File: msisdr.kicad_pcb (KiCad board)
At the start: 2 copper layers, 46.3 x 90.7 mm, 82 parts, among them J1 VCC_GPIO, J10 SMA_VHF1, J11 USB_OTG, J2 GPIO0, J3 GPIO1, J4 GPIO2, J5 GPIO3, J6 SMA_0_30MHZ, J7 SMA_30_60MHZ, J8 SMA_VHF2, J9 SMA_UHF, U1 msi2500, U2 msi001, U3 RT9193-28, U4 AP7313-30SAG, Y1 24MHz, Y2 24MHZ

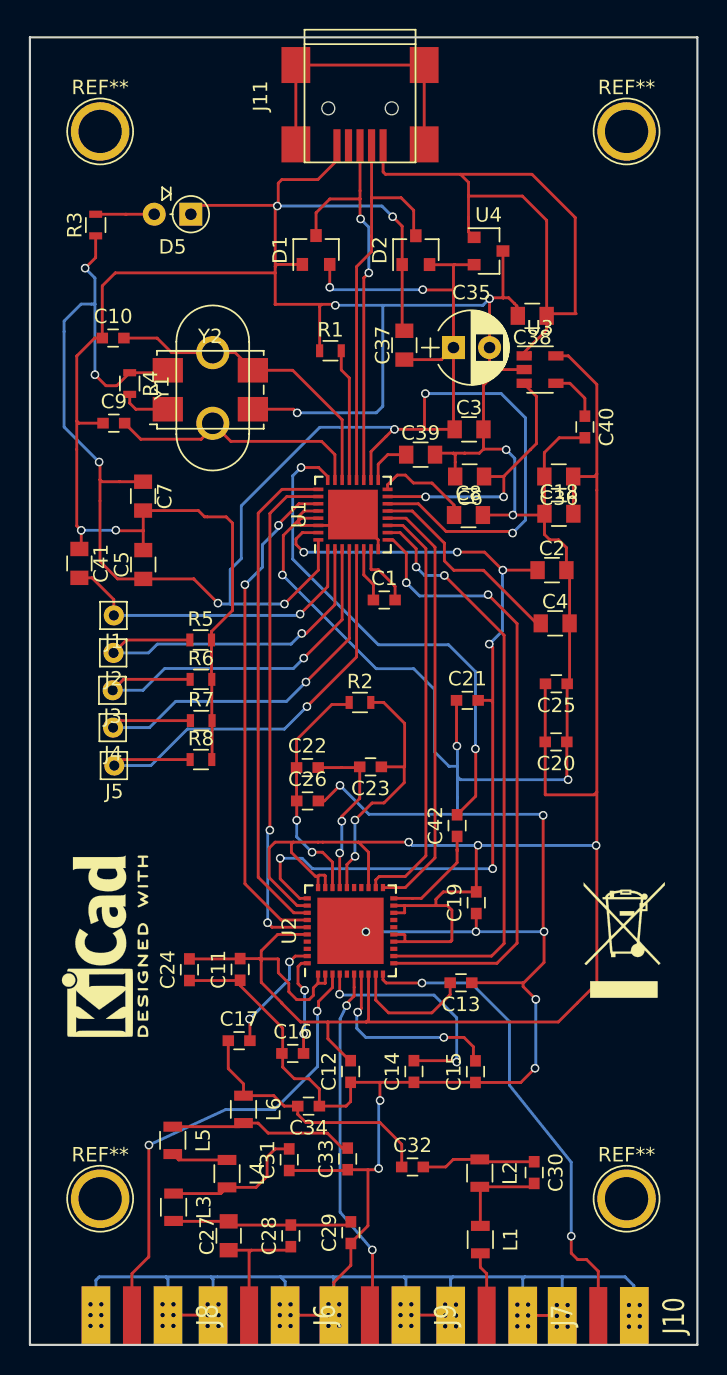
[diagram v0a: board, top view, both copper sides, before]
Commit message: finish route and output gerber file
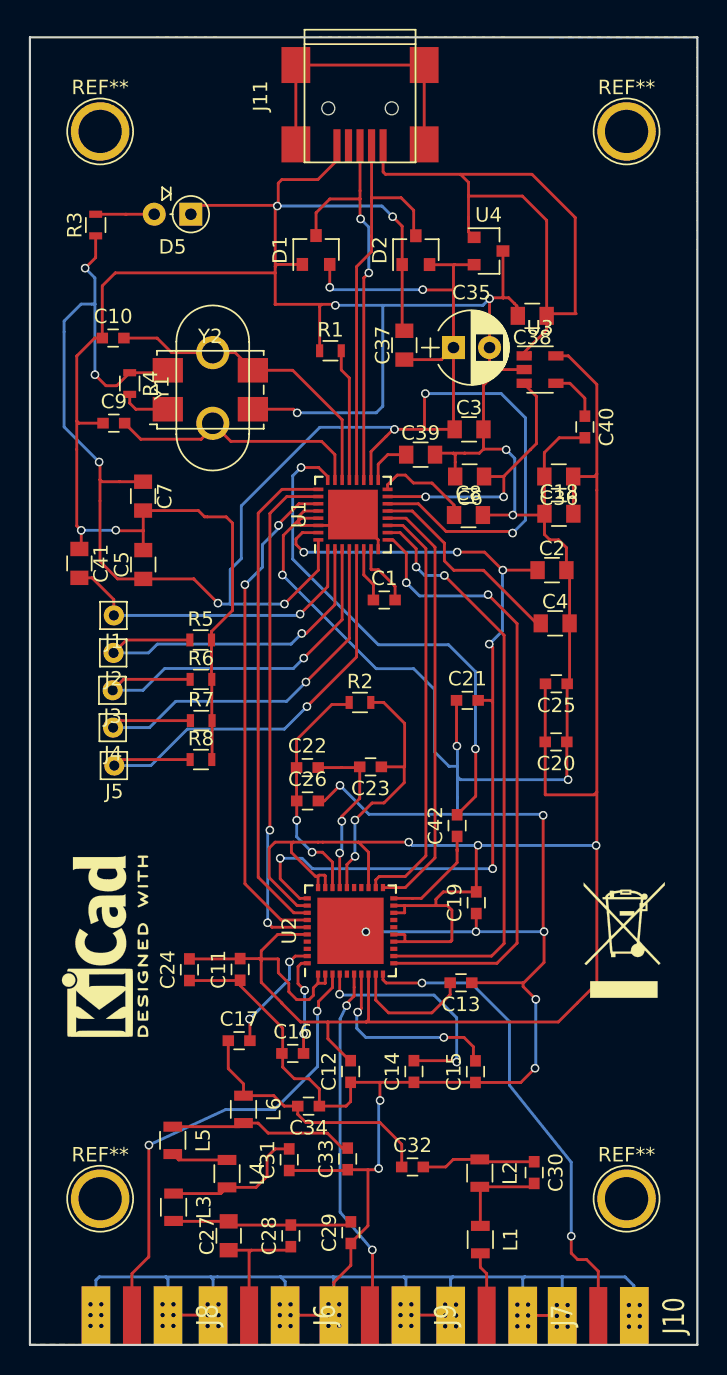
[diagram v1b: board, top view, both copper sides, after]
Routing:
- added copper zone on B.Cu, net GND
- added copper zone on F.Cu, net GND
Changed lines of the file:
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@@
     (visible_elements 7FFEFFFF)
     (pcbplotparams
-      (layerselection 0x00030_80000001)
+      (layerselection 0x01fff_80000001)
       (usegerberextensions false)
       (excludeedgelayer true)
@@
       (outputformat 1)
       (mirror false)
-      (drillshape 1)
+      (drillshape 0)
       (scaleselection 1)
-      (outputdirectory ""))
+      (outputdirectory gerber/))
   )
   (net 0 "")
@@
   (segment (start 125.01 71.34) (end 120.813 71.34) (width 0.2) (layer F.Cu) (net 7))
   (segment (start 125.799 70.226) (end 125.809 70.236) (width 0.2) (layer F.Cu) (net 7))
-  (segment (start 144.079 102.726) (end 144.079 99.611) (width 0.2) (layer F.Cu) (net 8) (status 400000))
+  (segment (start 144.079 102.726) (end 144.079 99.611) (width 0.2) (layer F.Cu) (net 8))
   (segment (start 144.14 99.43) (end 144.14 99.506) (width 0.2) (layer B.Cu) (net 8))
   (segment (start 144.184 99.474) (end 144.14 99.43) (width 0.2) (layer B.Cu) (net 8))
@@
   (segment (start 142.75 100.7) (end 140.274 103.176) (width 0.2) (layer F.Cu) (net 22))
   (segment (start 142.75 99.9) (end 142.75 99.78) (width 0.2) (layer F.Cu) (net 22))
-  (segment (start 142.75 99.78) (end 142.75 98.88) (width 0.2) (layer F.Cu) (net 22) (status 800000))
+  (segment (start 142.75 99.78) (end 142.75 98.88) (width 0.2) (layer F.Cu) (net 22))
   (segment (start 132.359 104.176) (end 131.429 104.176) (width 0.2) (layer F.Cu) (net 23))
   (segment (start 130.609 74.816) (end 133.129 74.816) (width 0.2) (layer F.Cu) (net 23))
@@
   (segment (start 123.09094 123.64208) (end 126.36762 123.64208) (width 0.2) (layer F.Cu) (net 33))
   (segment (start 126.36762 123.64208) (end 126.7968 123.2129) (width 0.2) (layer F.Cu) (net 33))
-  (segment (start 116.689 77.656) (end 116.689 78.821) (width 0.2) (layer F.Cu) (net 34) (status 800000))
-  (segment (start 116.689 78.821) (end 116.56 78.95) (width 0.2) (layer F.Cu) (net 34) (status C00000))
+  (segment (start 116.689 77.656) (end 116.689 78.821) (width 0.2) (layer F.Cu) (net 34))
+  (segment (start 116.689 78.821) (end 116.56 78.95) (width 0.2) (layer F.Cu) (net 34))
   (segment (start 138.94 59.23) (end 138.94 63.67) (width 0.2) (layer F.Cu) (net 34))
   (segment (start 138.94 63.67) (end 139.09 63.82) (width 0.2) (layer F.Cu) (net 34))
@@
   (segment (start 120.05 68.84) (end 120.05 68.23) (width 0.2) (layer F.Cu) (net 61))
   (segment (start 120.47 69.26) (end 120.05 68.84) (width 0.2) (layer F.Cu) (net 61))
-  (segment (start 116.56 80.95) (end 117.44 80.95) (width 0.2) (layer F.Cu) (net 62) (status 400000))
-  (segment (start 118.949 82.459) (end 118.949 83.556) (width 0.2) (layer F.Cu) (net 62) (status 800000))
+  (segment (start 116.56 80.95) (end 117.44 80.95) (width 0.2) (layer F.Cu) (net 62))
+  (segment (start 118.949 82.459) (end 118.949 83.556) (width 0.2) (layer F.Cu) (net 62))
   (segment (start 117.44 80.95) (end 118.949 82.459) (width 0.2) (layer F.Cu) (net 62))
   (segment (start 118.949 83.556) (end 131.779 83.556) (width 0.2) (layer B.Cu) (net 62))
@@
   (via (at 131.869 83.466) (size 0.6) (drill 0.4) (layers F.Cu B.Cu) (net 62))
   (segment (start 131.779 83.556) (end 131.869 83.466) (width 0.2) (layer B.Cu) (net 62))
-  (segment (start 133.779 74.166) (end 133.779 73.929) (width 0.2) (layer F.Cu) (net 63) (status C00000))
-  (segment (start 133.779 73.929) (end 133.15 73.3) (width 0.2) (layer F.Cu) (net 63) (status 400000))
+  (segment (start 133.779 74.166) (end 133.779 73.929) (width 0.2) (layer F.Cu) (net 63))
+  (segment (start 133.779 73.929) (end 133.15 73.3) (width 0.2) (layer F.Cu) (net 63))
   (segment (start 133.15 73.3) (end 131.93 73.3) (width 0.2) (layer F.Cu) (net 63))
   (via (at 131.93 73.3) (size 0.6) (drill 0.4) (layers F.Cu B.Cu) (net 63))
@@
   (segment (start 144.02 92.81) (end 144.04 92.83) (width 0.2) (layer F.Cu) (net 63))
   (segment (start 144.04 92.83) (end 144.04 96.09) (width 0.2) (layer F.Cu) (net 63))
-  (segment (start 144.04 96.09) (end 142.75 97.38) (width 0.2) (layer F.Cu) (net 63) (status 800000))
+  (segment (start 144.04 96.09) (end 142.75 97.38) (width 0.2) (layer F.Cu) (net 63))
+  (zone (net 34) (net_name GND) (layer F.Cu) (hatch edge 0.508)
+    (connect_pads (clearance 0.508))
+    (min_thickness 0.254)
+    (fill yes (arc_segments 16) (thermal_gap 0.508) (thermal_bridge_width 0.508))
+    (polygon
+      (pts
+        (xy 113.16 43.47) (xy 113.15 134.1) (xy 159.41 134.12) (xy 159.39 43.46) (xy 113.17 43.47)
+      )
+    )
+  )
+  (zone (net 34) (net_name GND) (layer B.Cu) (hatch edge 0.508)
+    (connect_pads (clearance 0.508))
+    (min_thickness 0.254)
+    (fill yes (arc_segments 16) (thermal_gap 0.508) (thermal_bridge_width 0.508))
+    (polygon
+      (pts
+        (xy 159.38 43.48) (xy 159.4 134.12) (xy 113.13 134.12) (xy 113.16 43.47)
+      )
+    )
+  )
 )
